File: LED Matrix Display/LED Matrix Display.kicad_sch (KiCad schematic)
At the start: 56 parts, among them J1 I2C Sensor 1, J2 LED Display, J3 Prodrammer, J4 12V, J5 SW, J6 Charger, SW1 BOOT, SW2 RESET, SW3 SW_Reed, U1 ESP32-WROOM-E, U2 BME280, U3 LM2596S-5, U4 AMS1117-3.3

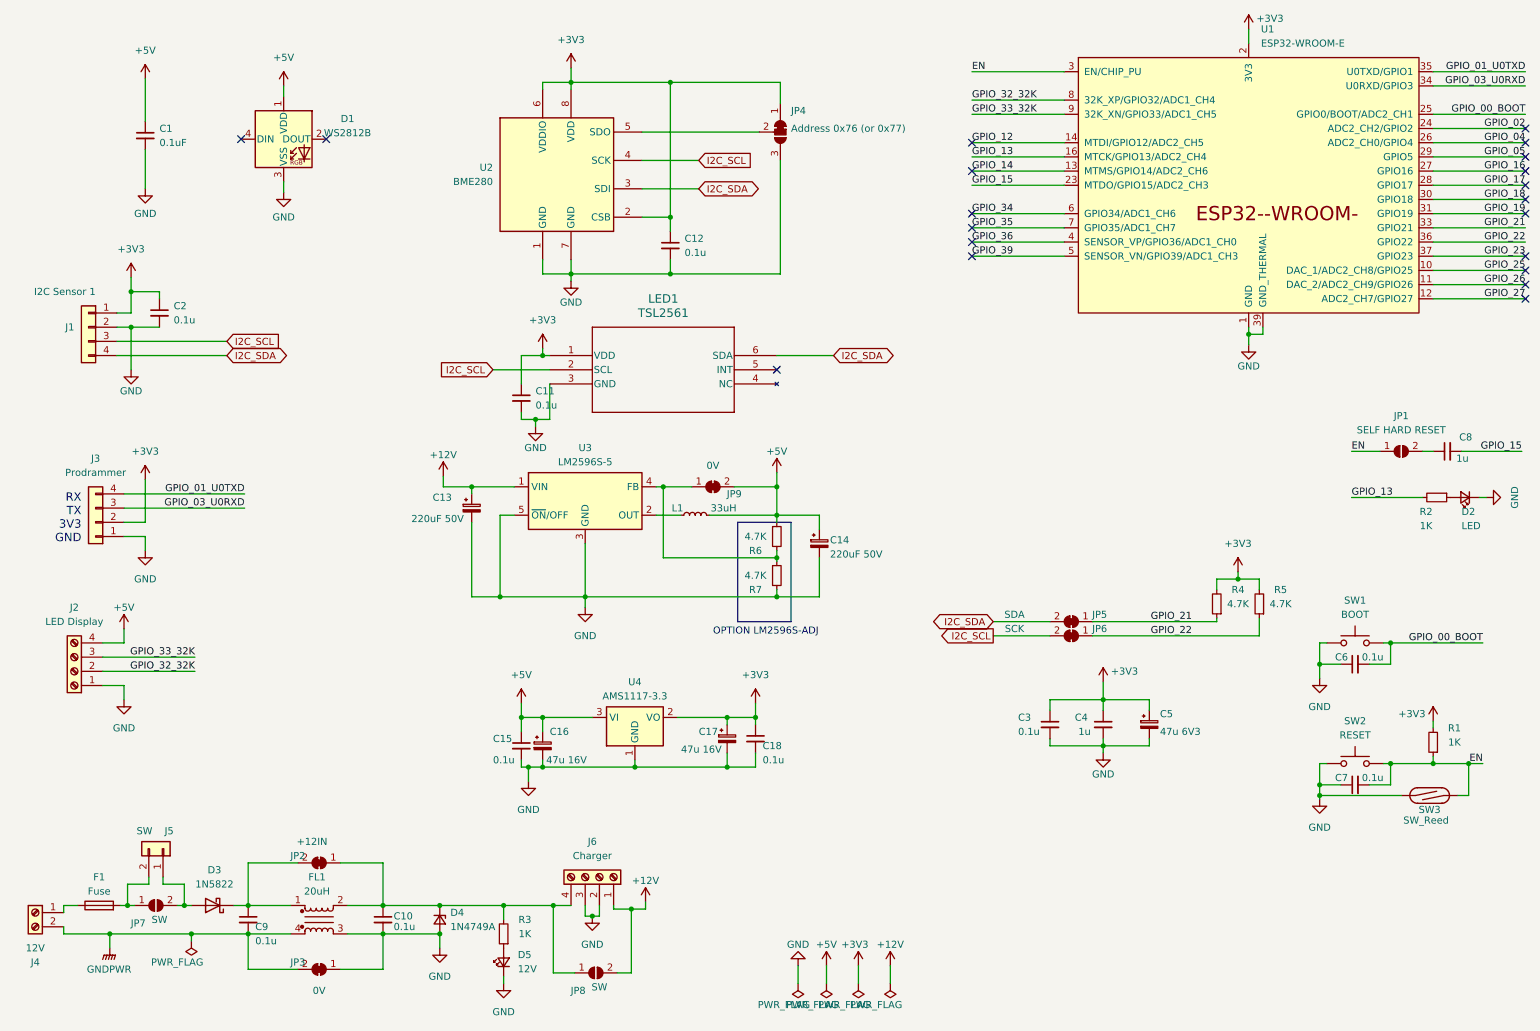
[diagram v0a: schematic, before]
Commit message: LED
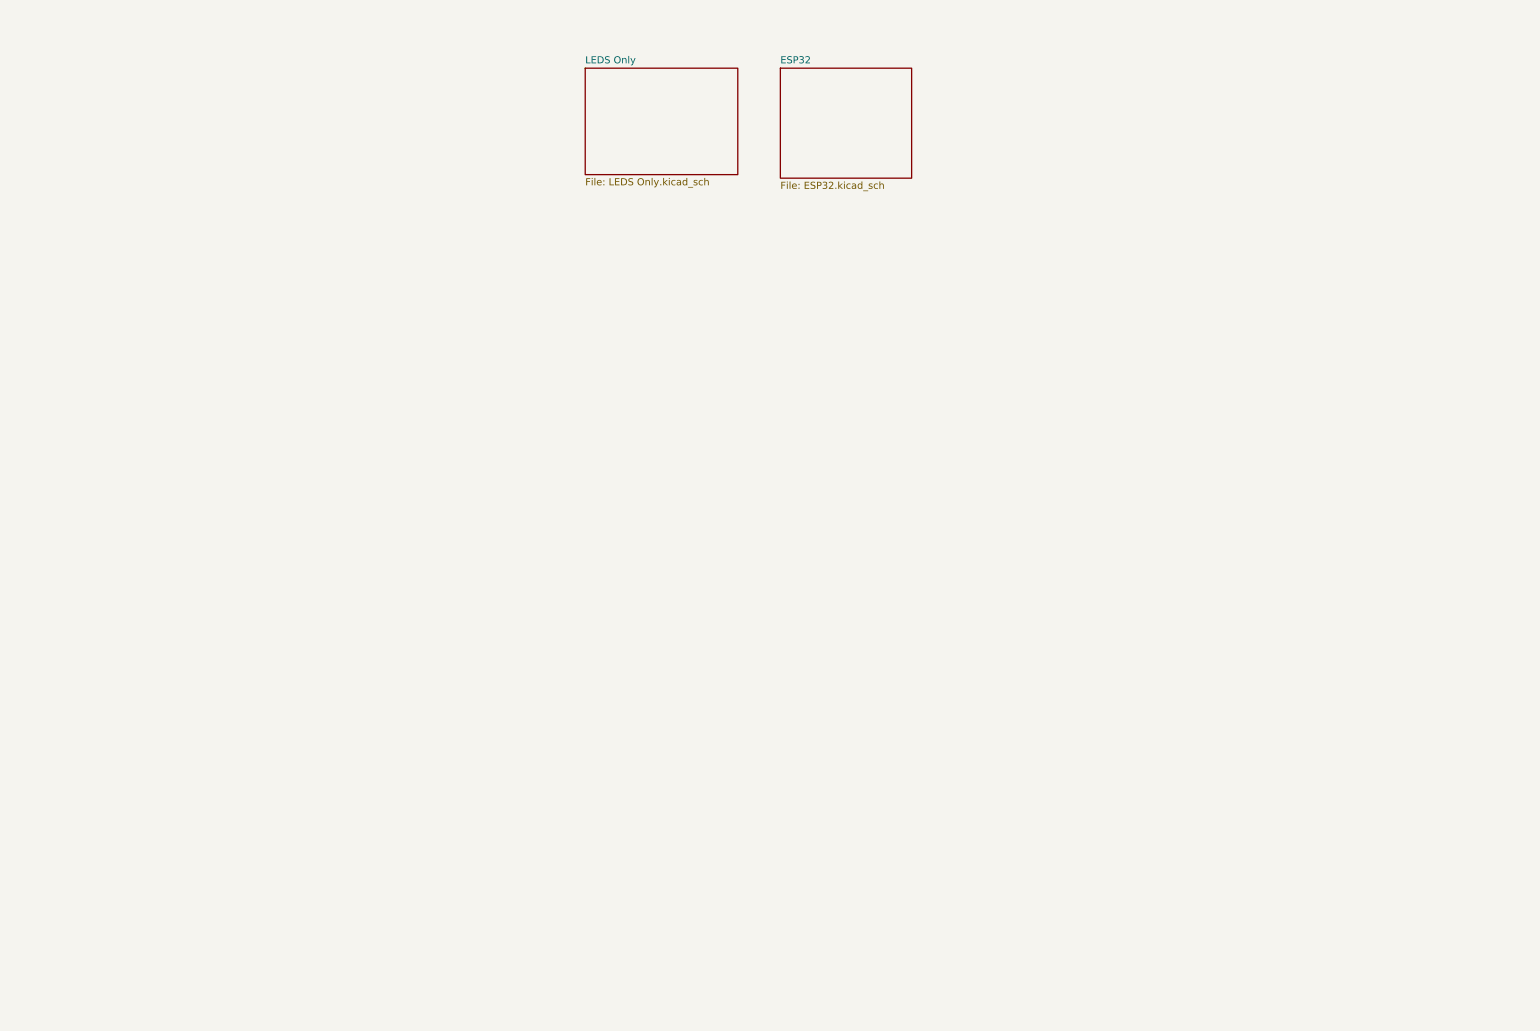
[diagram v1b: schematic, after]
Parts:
- removed C1: 0.1uF, Capacitor_SMD:C_0402_1005Metric, symbol Device:C_Small
- removed C10, C11, C12, C15, C18, C2, C3, C6, C7, C9: 0.1u, Capacitor_SMD:C_0805_2012Metric_Pad1.18x1.45mm_HandSolder, symbol Device:C_Small
- removed C13, C14: 220uF 50V, Capacitor_SMD:CP_Elec_5x5.8, symbol Device:C_Polarized_Small
- removed C16, C17: 47u 16V, Capacitor_SMD:CP_Elec_5x5.8, symbol Device:C_Polarized_Small
- removed C4, C8: 1u, Capacitor_SMD:C_0805_2012Metric_Pad1.18x1.45mm_HandSolder, symbol Device:C_Small
- removed C5: 47u 6V3, Capacitor_Tantalum_SMD:CP_EIA-3528-21_Kemet-B_Pad1.50x2.35mm_HandSolder, symbol Device:C_Polarized_Small
- removed D1: WS2812B, LED_SMD:LED_WS2812B_PLCC4_5.0x5.0mm_P3.2mm, symbol LED:WS2812B
- removed D2: LED, LED_SMD:LED_0805_2012Metric_Pad1.15x1.40mm_HandSolder, symbol Device:LED_Small
- removed D3: 1N5822, Diode_SMD:D_SMC, symbol Diode:1N5822
- removed D4: 1N4749A, Diode_SMD:D_SMA, symbol Device:D_Zener_Small
- removed D5: 12V, LED_SMD:LED_0805_2012Metric_Pad1.15x1.40mm_HandSolder, symbol Device:LED_Small
- removed F1: Fuse, Fuse:Fuse_1812_4532Metric, symbol Device:Fuse
- removed FL1: 20uH, Transformer_SMD:Pulse_PA2001NL, symbol Device:Filter_EMI_CommonMode
- removed J1: I2C Sensor 1, Connector_JST:JST_PH_S4B-PH-SM4-TB_1x04-1MP_P2.00mm_Horizontal, symbol Connector_Generic:Conn_01x04
- removed J2: LED Display, Connector_Molex:Molex_Micro-Fit_3.0_43650-0410_1x04-1MP_P3.00mm_Horizontal_PnP, symbol Connector:Screw_Terminal_01x04
- removed J3: Prodrammer, Connector_JST:JST_PH_S4B-PH-SM4-TB_1x04-1MP_P2.00mm_Horizontal, symbol Connector_Generic:Conn_01x04
- removed J4: 12V, Connector_Molex:Molex_Micro-Fit_3.0_43650-0210_1x02-1MP_P3.00mm_Horizontal_PnP, symbol Connector:Screw_Terminal_01x02
- removed J5: SW, Connector_Molex:Molex_Micro-Fit_3.0_43650-0210_1x02-1MP_P3.00mm_Horizontal_PnP, symbol Connector_Generic:Conn_01x02
- removed J6: Charger, Connector_Molex:Molex_Micro-Fit_3.0_43650-0410_1x04-1MP_P3.00mm_Horizontal_PnP, symbol Connector:Screw_Terminal_01x04
- removed JP1: SELF HARD RESET, Jumper:SolderJumper-2_P1.3mm_Open_RoundedPad1.0x1.5mm, symbol Jumper:SolderJumper_2_Open
- removed JP2: +12IN, 1Display:NOSILK SolderJumper-2_P1.3mm_Open_Pad1.0x1.5mm, symbol Jumper:SolderJumper_2_Bridged
- removed JP3, JP9: 0V, 1Display:NOSILK SolderJumper-2_P1.3mm_Open_Pad1.0x1.5mm, symbol Jumper:SolderJumper_2_Bridged
- removed JP4: Address 0x76 (or 0x77), Jumper:SolderJumper-3_P1.3mm_Bridged12_Pad1.0x1.5mm, symbol Jumper:SolderJumper_3_Bridged12
- removed JP5: SDA, Jumper:SolderJumper-2_P1.3mm_Bridged_Pad1.0x1.5mm, symbol Jumper:SolderJumper_2_Bridged
- removed JP6: SCK, Jumper:SolderJumper-2_P1.3mm_Bridged_Pad1.0x1.5mm, symbol Jumper:SolderJumper_2_Bridged
- removed JP7, JP8: SW, Jumper:SolderJumper-2_P1.3mm_Open_RoundedPad1.0x1.5mm, symbol Jumper:SolderJumper_2_Open
- removed L1: 33uH, Inductor_SMD:L_12x12mm_H4.5mm, symbol Device:L_Small
- removed LED1: TSL2561, 1Display:TSL2561, symbol 1Display2:TSL25723FN
- removed R1, R2, R3: 1K, Resistor_SMD:R_0805_2012Metric_Pad1.20x1.40mm_HandSolder, symbol Device:R_Small
- removed R4, R5, R6, R7: 4.7K, Resistor_SMD:R_0805_2012Metric_Pad1.20x1.40mm_HandSolder, symbol Device:R_Small
- removed SW1: BOOT, Button_Switch_SMD:SW_Push_1P1T_NO_6x6mm_H9.5mm, symbol Switch:SW_Push
- removed SW2: RESET, Button_Switch_SMD:SW_Push_1P1T_NO_6x6mm_H9.5mm, symbol Switch:SW_Push
- removed SW3: SW_Reed, Button_Switch_SMD:SW_SPST_REED_CT05-XXXX-J1, symbol Switch:SW_Reed
- removed U1: ESP32-WROOM-E, PCM_Espressif:ESP32-WROOM-32E, symbol PCM_Espressif:ESP32-WROOM-E
- removed U2: BME280, Package_LGA:Bosch_LGA-8_2.5x2.5mm_P0.65mm_ClockwisePinNumbering, symbol Sensor:BME280
- removed U3: LM2596S-5, Package_TO_SOT_SMD:TO-263-5_TabPin3, symbol Regulator_Switching:LM2596S-5
- removed U4: AMS1117-3.3, Package_TO_SOT_SMD:SOT-223-3_TabPin2, symbol Regulator_Linear:AMS1117-5.0
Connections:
- no-connect marks 20 -> 0
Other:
- added sheet ESP32 (ESP32.kicad_sch)
- added sheet LEDS Only (LEDS Only.kicad_sch)
- note removed: "OPTION LM2596S-ADJ"
- note removed: "RX TX 3V3 GND"

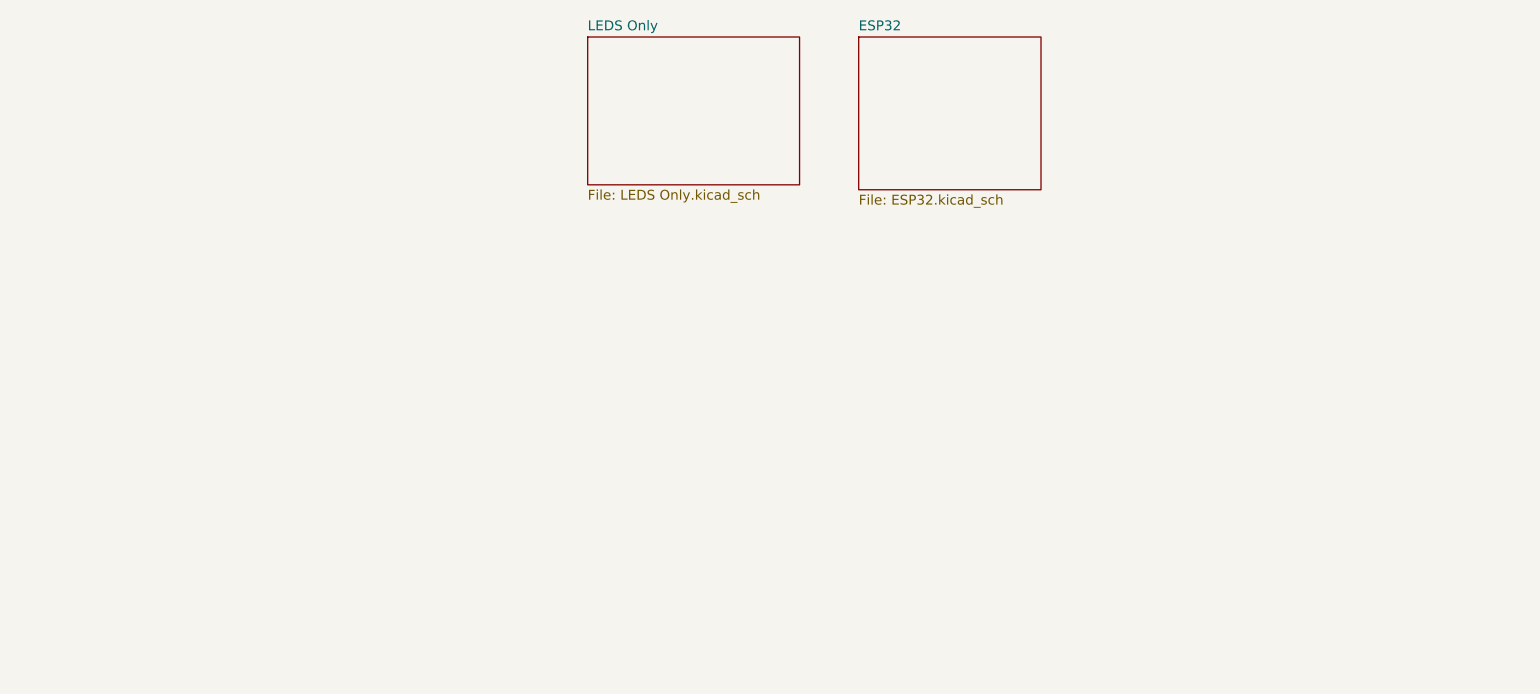
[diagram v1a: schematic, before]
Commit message: LED MX Release candidate
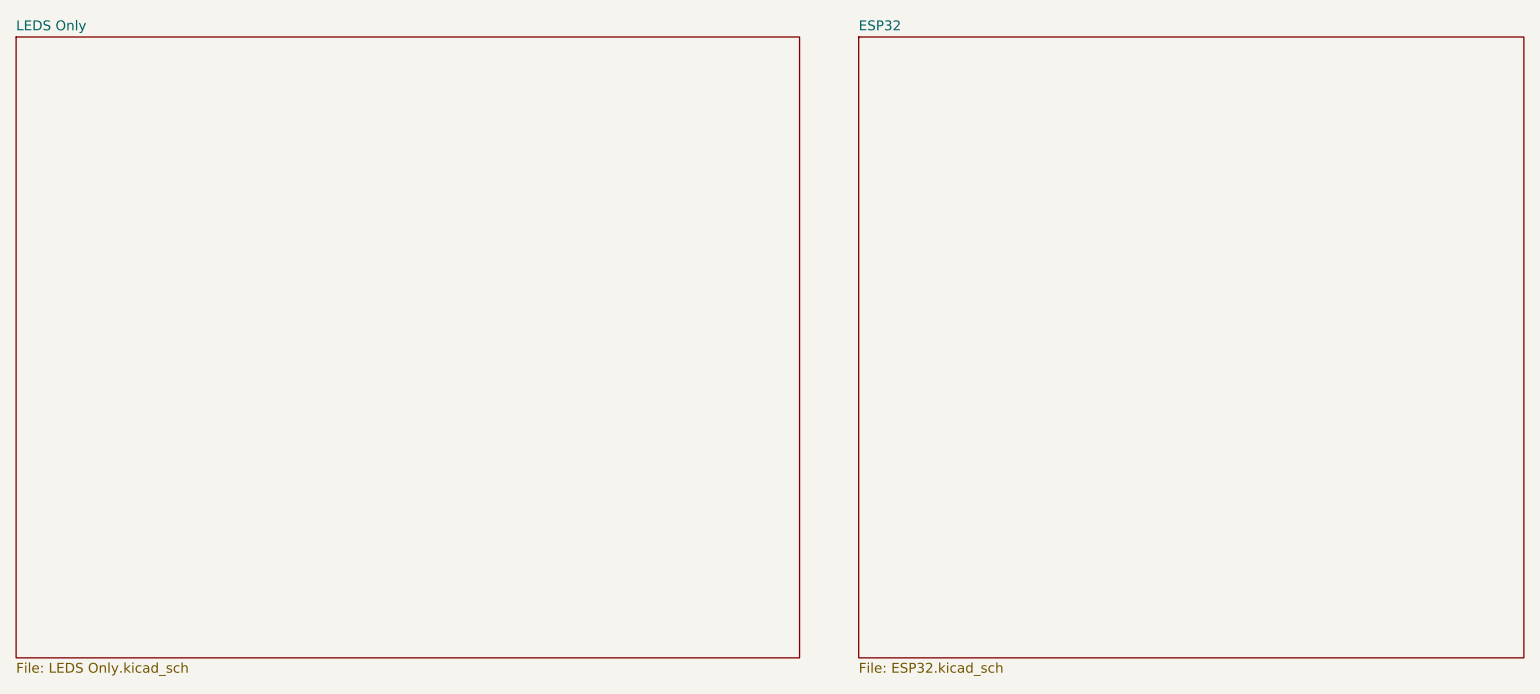
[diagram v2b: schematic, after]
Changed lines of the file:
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@@
 (kicad_sch (version 20230121) (generator eeschema)
   (paper "A4")
-  (sheet (at 149.225 24.13) (size 23.495 19.685) (fields_autoplaced)
+  (sheet (at 149.225 24.13) (size 85.725 80.01) (fields_autoplaced)
     (stroke (width 0.1524) (type solid))
     (fill (color 0 0 0 0.0000))
@@
       (effects (font (size 1.27 1.27)) (justify left bottom))
     )
-    (property "Sheetfile" "ESP32.kicad_sch" (at 149.225 44.3996 0)
+    (property "Sheetfile" "ESP32.kicad_sch" (at 149.225 104.7246 0)
       (effects (font (size 1.27 1.27)) (justify left top))
     )
@@
     )
   )
-  (sheet (at 114.3 24.13) (size 27.305 19.05) (fields_autoplaced)
+  (sheet (at 40.64 24.13) (size 100.965 80.01) (fields_autoplaced)
     (stroke (width 0.1524) (type solid))
     (fill (color 0 0 0 0.0000))
-    (property "Sheetname" "LEDS Only" (at 114.3 23.4184 0)
+    (property "Sheetname" "LEDS Only" (at 40.64 23.4184 0)
       (effects (font (size 1.27 1.27)) (justify left bottom))
     )
-    (property "Sheetfile" "LEDS Only.kicad_sch" (at 114.3 43.7646 0)
+    (property "Sheetfile" "LEDS Only.kicad_sch" (at 40.64 104.7246 0)
       (effects (font (size 1.27 1.27)) (justify left top))
     )
-    (property "Field2" "" (at 114.3 24.13 0)
+    (property "Field2" "" (at 40.64 24.13 0)
       (effects (font (size 1.27 1.27)) hide)
     )
